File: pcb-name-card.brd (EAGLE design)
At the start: 87.5 x 53.3 mm, 7 parts

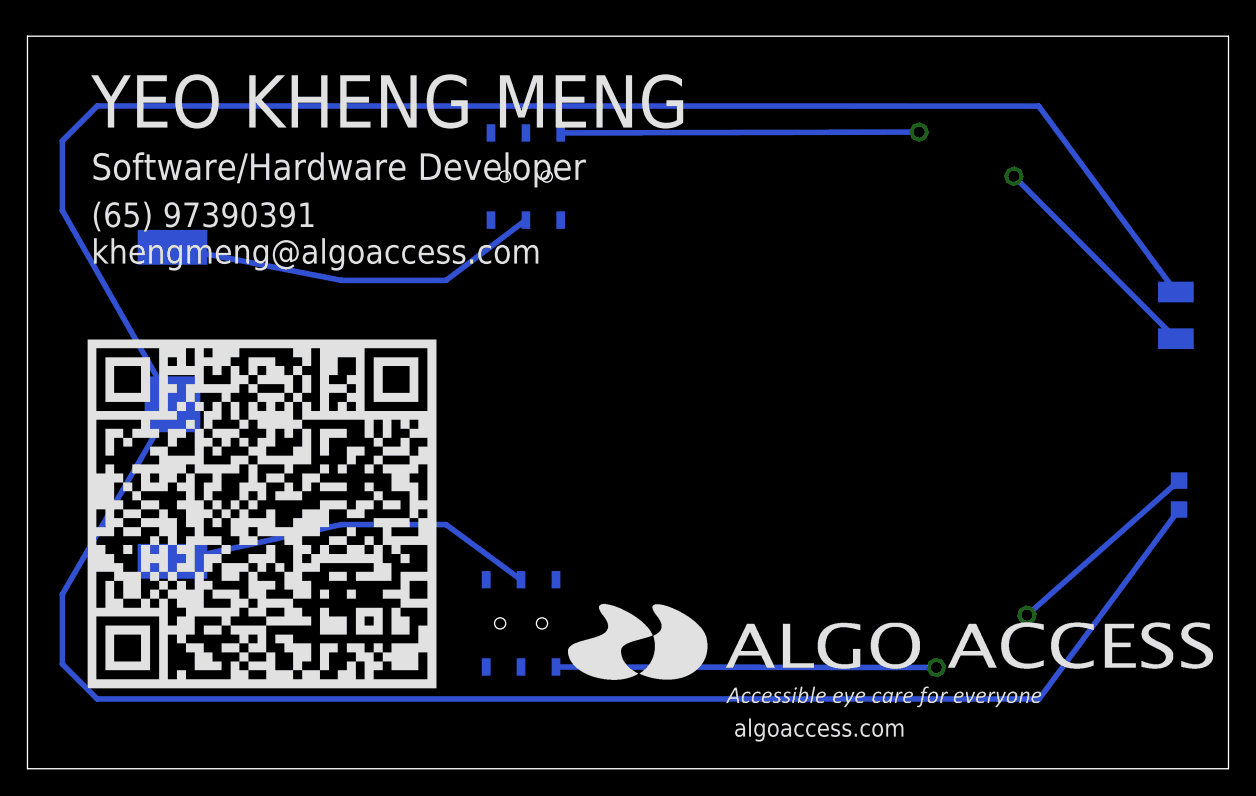
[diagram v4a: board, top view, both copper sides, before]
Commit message: more changes
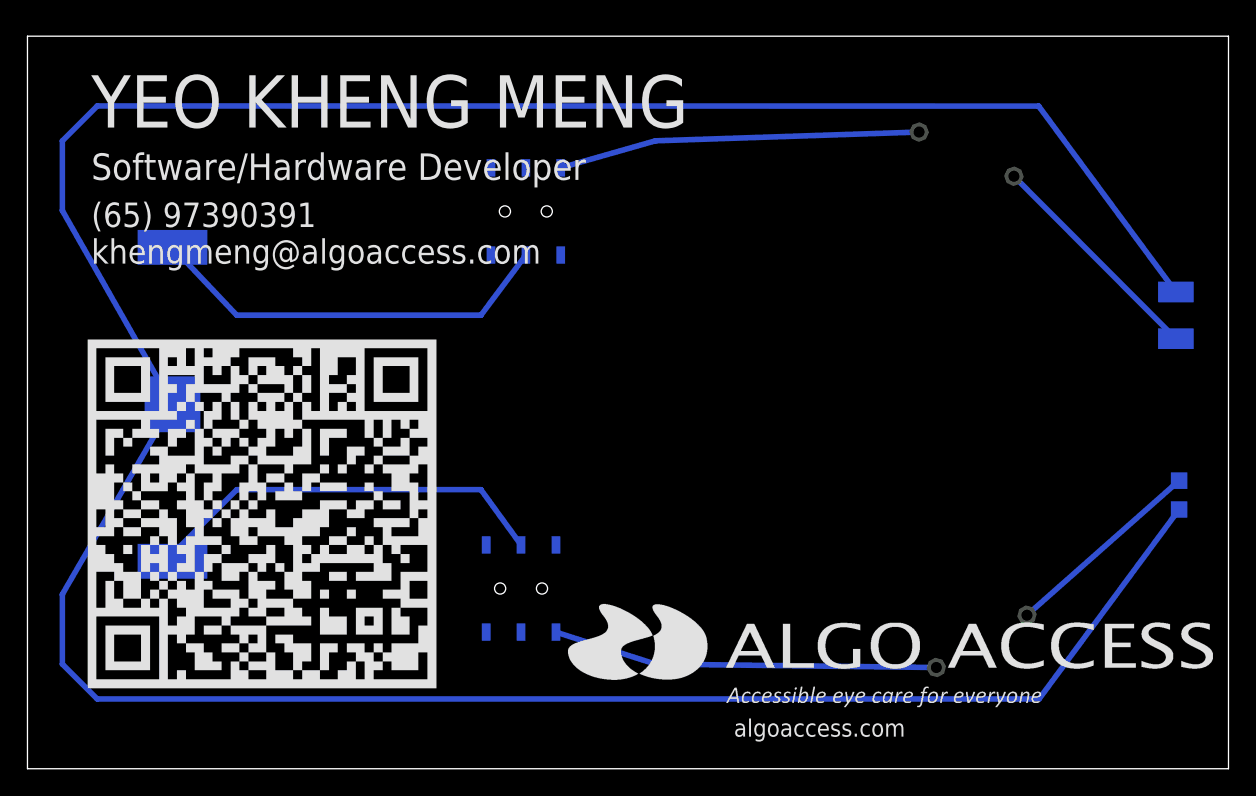
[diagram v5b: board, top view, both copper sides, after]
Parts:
- moved SW1 2.54 mm to (36.3, 40.6)
- moved SW2 2.54 mm to (35.9, 13.1)
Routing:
- net N$7: track 27.0 -> 30.4 mm
- net N$3: track 27.4 -> 30.1 mm
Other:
- board text added: "Rev 1"
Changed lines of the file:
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@@
 <grid distance="0.1" unitdist="inch" unit="inch" style="lines" multiple="1" display="yes" altdistance="0.025" altunitdist="inch" altunit="inch"/>
 <layers>
-<layer number="1" name="Top" color="4" fill="1" visible="yes" active="yes"/>
+<layer number="1" name="Top" color="4" fill="1" visible="no" active="yes"/>
 <layer number="2" name="Route2" color="1" fill="3" visible="no" active="no"/>
 <layer number="3" name="Route3" color="4" fill="3" visible="no" active="no"/>
@@
 <layer number="19" name="Unrouted" color="6" fill="1" visible="yes" active="yes"/>
 <layer number="20" name="Dimension" color="15" fill="1" visible="yes" active="yes"/>
-<layer number="21" name="tPlace" color="7" fill="1" visible="yes" active="yes"/>
+<layer number="21" name="tPlace" color="7" fill="1" visible="no" active="yes"/>
 <layer number="22" name="bPlace" color="7" fill="1" visible="yes" active="yes"/>
-<layer number="23" name="tOrigins" color="15" fill="1" visible="yes" active="yes"/>
+<layer number="23" name="tOrigins" color="15" fill="1" visible="no" active="yes"/>
 <layer number="24" name="bOrigins" color="15" fill="1" visible="yes" active="yes"/>
-<layer number="25" name="tNames" color="7" fill="1" visible="yes" active="yes"/>
+<layer number="25" name="tNames" color="7" fill="1" visible="no" active="yes"/>
 <layer number="26" name="bNames" color="7" fill="1" visible="yes" active="yes"/>
-<layer number="27" name="tValues" color="7" fill="1" visible="yes" active="yes"/>
+<layer number="27" name="tValues" color="7" fill="1" visible="no" active="yes"/>
 <layer number="28" name="bValues" color="7" fill="1" visible="yes" active="yes"/>
 <layer number="29" name="tStop" color="7" fill="3" visible="no" active="yes"/>
@@
 <layer number="119" name="KAP_TEKEN" color="7" fill="1" visible="no" active="no"/>
 <layer number="120" name="KAP_MAAT1" color="7" fill="1" visible="no" active="no"/>
-<layer number="121" name="_tsilk" color="7" fill="1" visible="yes" active="yes"/>
+<layer number="121" name="_tsilk" color="7" fill="1" visible="no" active="yes"/>
 <layer number="122" name="_bsilk" color="7" fill="1" visible="yes" active="yes"/>
 <layer number="123" name="tTestmark" color="7" fill="1" visible="no" active="yes"/>
@@
 before toggling the switches</text>
 <text x="12.7" y="10.16" size="1.4224" layer="22" rot="MR0">CR2025</text>
+<text x="10.16" y="2.54" size="1.27" layer="22" rot="MR0">Rev 1</text>
 </plain>
 <attributes>
@@
 <attribute name="VALUE" x="22.908778125" y="30.852109375" size="1.6764" layer="28" font="vector" rot="MR270"/>
 </element>
-<element name="SW1" library="Seeed-OPL-Switch" package="SW6-2.54-SMD-7.0X3.5X1.5MM" value="" x="36.288984375" y="43.120309375" smashed="yes" rot="MR90">
-<attribute name="MPN" value="MS-22C01" x="36.288984375" y="43.120309375" size="1.778" layer="28" rot="MR90" display="off"/>
-<attribute name="NAME" x="36.695384375" y="44.441109375" size="0.889" layer="26" ratio="11" rot="MR270"/>
-<attribute name="VALUE" x="31.589984375" y="41.215309375" size="0.889" layer="28" ratio="11" rot="MR90"/>
+<element name="SW1" library="Seeed-OPL-Switch" package="SW6-2.54-SMD-7.0X3.5X1.5MM" value="" x="36.288984375" y="40.580309375" smashed="yes" rot="MR90">
+<attribute name="MPN" value="MS-22C01" x="36.288984375" y="40.580309375" size="1.778" layer="28" rot="MR90" display="off"/>
+<attribute name="NAME" x="36.695384375" y="41.901109375" size="0.889" layer="26" ratio="11" rot="MR270"/>
+<attribute name="VALUE" x="31.589984375" y="38.675309375" size="0.889" layer="28" ratio="11" rot="MR90"/>
 </element>
-<element name="SW2" library="Seeed-OPL-Switch" package="SW6-2.54-SMD-7.0X3.5X1.5MM" value="" x="35.941" y="10.5829125" smashed="yes" rot="MR90">
-<attribute name="MPN" value="MS-22C01" x="35.941" y="10.5829125" size="1.778" layer="28" rot="MR90" display="off"/>
-<attribute name="NAME" x="36.4998" y="11.8021125" size="0.889" layer="26" ratio="11" rot="MR270"/>
-<attribute name="VALUE" x="31.242" y="8.6779125" size="0.889" layer="28" ratio="11" rot="MR90"/>
+<element name="SW2" library="Seeed-OPL-Switch" package="SW6-2.54-SMD-7.0X3.5X1.5MM" value="" x="35.941" y="13.1229125" smashed="yes" rot="MR90">
+<attribute name="MPN" value="MS-22C01" x="35.941" y="13.1229125" size="1.778" layer="28" rot="MR90" display="off"/>
+<attribute name="NAME" x="36.4998" y="14.3421125" size="0.889" layer="26" ratio="11" rot="MR270"/>
+<attribute name="VALUE" x="31.242" y="11.2179125" size="0.889" layer="28" ratio="11" rot="MR90"/>
 </element>
 <element name="R1" library="resistor" package="0207/7" value="" x="68.3768" y="44.74971875" smashed="yes" rot="MR25">
@@
 <contactref element="U$1" pad="+$1"/>
 <contactref element="SW1" pad="COM1"/>
-<wire x1="10.558778125" y1="37.964109375" x2="22.86" y2="35.56" width="0.4064" layer="16"/>
-<wire x1="22.86" y1="35.56" x2="30.48" y2="35.56" width="0.4064" layer="16"/>
-<wire x1="30.48" y1="35.56" x2="36.288984375" y2="39.945309375" width="0.4064" layer="16"/>
+<wire x1="36.288984375" y1="37.405309375" x2="33.02" y2="33.02" width="0.4064" layer="16"/>
+<wire x1="33.02" y1="33.02" x2="15.24" y2="33.02" width="0.4064" layer="16"/>
+<wire x1="15.24" y1="33.02" x2="10.558778125" y2="37.964109375" width="0.4064" layer="16"/>
 </signal>
 <signal name="N$7">
 <contactref element="U$1" pad="+$2"/>
 <contactref element="SW2" pad="COM2"/>
-<wire x1="10.558778125" y1="15.104109375" x2="22.86" y2="17.78" width="0.4064" layer="16"/>
-<wire x1="22.86" y1="17.78" x2="30.48" y2="17.78" width="0.4064" layer="16"/>
-<wire x1="30.48" y1="17.78" x2="35.941" y2="13.7579125" width="0.4064" layer="16"/>
+<wire x1="35.941" y1="16.2979125" x2="33.02" y2="20.32" width="0.4064" layer="16"/>
+<wire x1="33.02" y1="20.32" x2="22.86" y2="20.32" width="0" layer="19" extent="1-16"/>
+<wire x1="10.558778125" y1="15.104109375" x2="10.16" y2="15.24" width="0.4064" layer="16"/>
+<wire x1="10.16" y1="15.24" x2="15.24" y2="20.32" width="0.4064" layer="16"/>
+<wire x1="15.24" y1="20.32" x2="33.02" y2="20.32" width="0.4064" layer="16"/>
 </signal>
 <signal name="N$5">
 <contactref element="R2" pad="2"/>
 <contactref element="SW2" pad="CH1A"/>
-<wire x1="66.179603125" y1="7.371075" x2="38.481" y2="7.4079125" width="0.4064" layer="16"/>
+<wire x1="38.481" y1="9.9479125" x2="45.72" y2="7.62" width="0.4064" layer="16"/>
+<wire x1="45.72" y1="7.62" x2="66.179603125" y2="7.371075" width="0.4064" layer="16"/>
 </signal>
 <signal name="N$4">
 <contactref element="R1" pad="2"/>
 <contactref element="SW1" pad="CH2A"/>
-<wire x1="64.92376875" y1="46.35989375" x2="38.828984375" y2="46.295309375" width="0.4064" layer="16"/>
+<wire x1="38.828984375" y1="43.755309375" x2="45.72" y2="45.72" width="0.4064" layer="16"/>
+<wire x1="45.72" y1="45.72" x2="64.92376875" y2="46.35989375" width="0.4064" layer="16"/>
 </signal>
 </signals>

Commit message: dimension
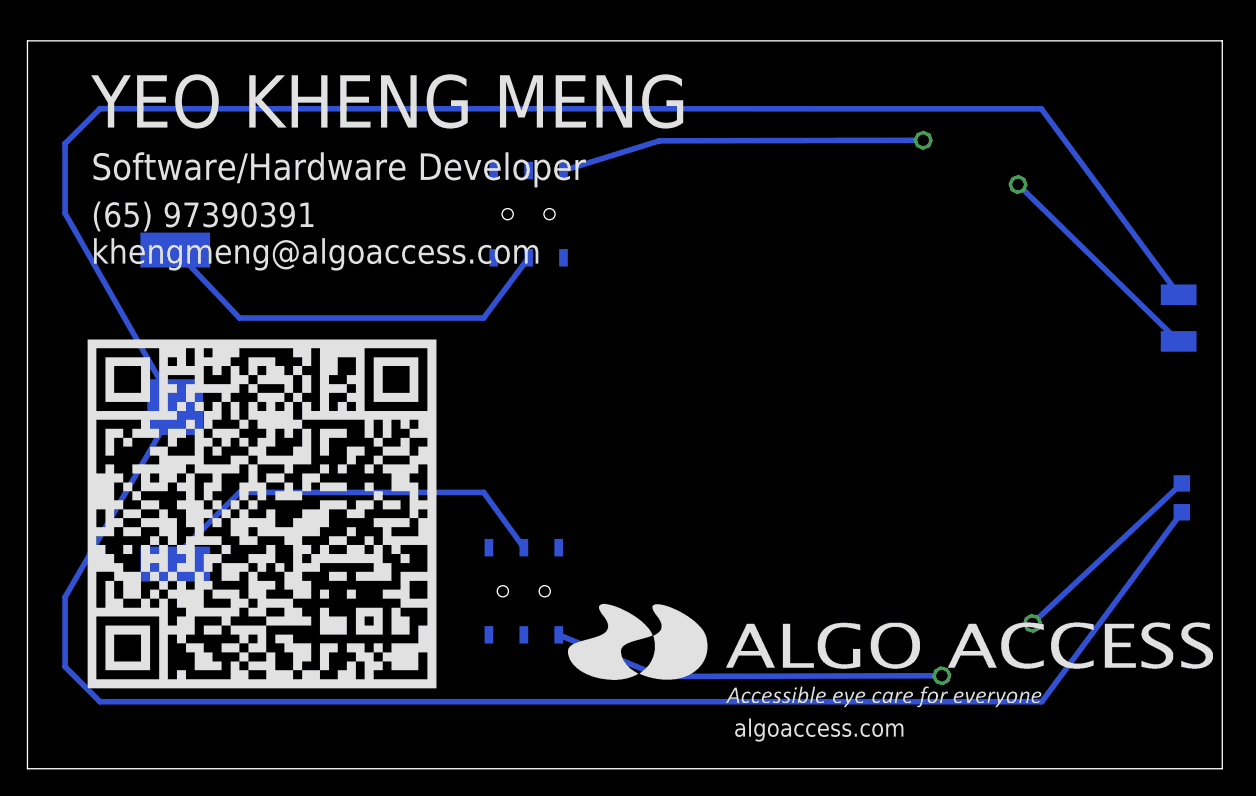
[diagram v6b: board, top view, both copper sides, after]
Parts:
- moved R2 0.72 mm to (69.9, 8.68)
- moved R1 0.67 mm to (68.7, 44.1)
- moved LED1 0.28 mm to (83.8, 32.8)
- moved SW1 0.28 mm to (36.5, 40.4)
- moved U$1 0.28 mm to (10.8, 26.3)
- moved SW2 0.28 mm to (36.1, 12.9)
- moved LED2 0.28 mm to (84.1, 19.7)
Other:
- board size 87.5 x 53.3 mm -> 87 x 53 mm
